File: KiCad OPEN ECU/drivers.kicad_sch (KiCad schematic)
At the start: 52 parts, among them SW5 SW_DPDT_x2, U3 TC4424A, U4 TC4424A, U5 MC33810, U6 MC33810, U7 TC4424A, U8 TC4424A

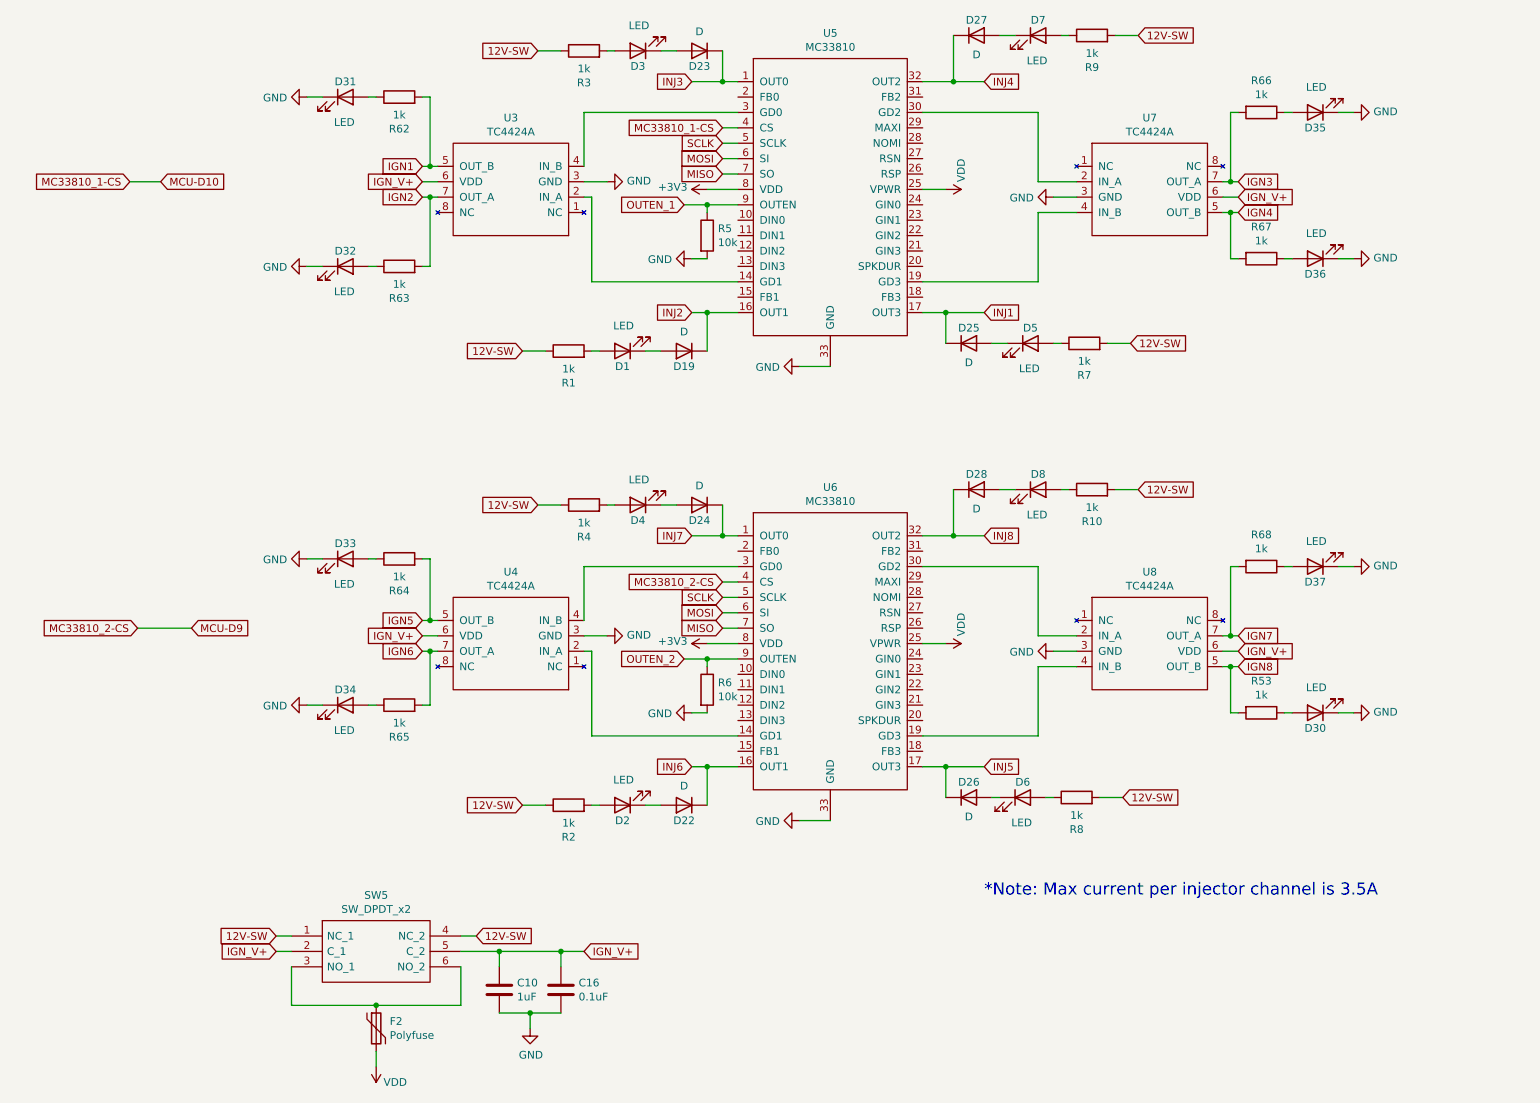
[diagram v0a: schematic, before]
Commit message: Add files via upload
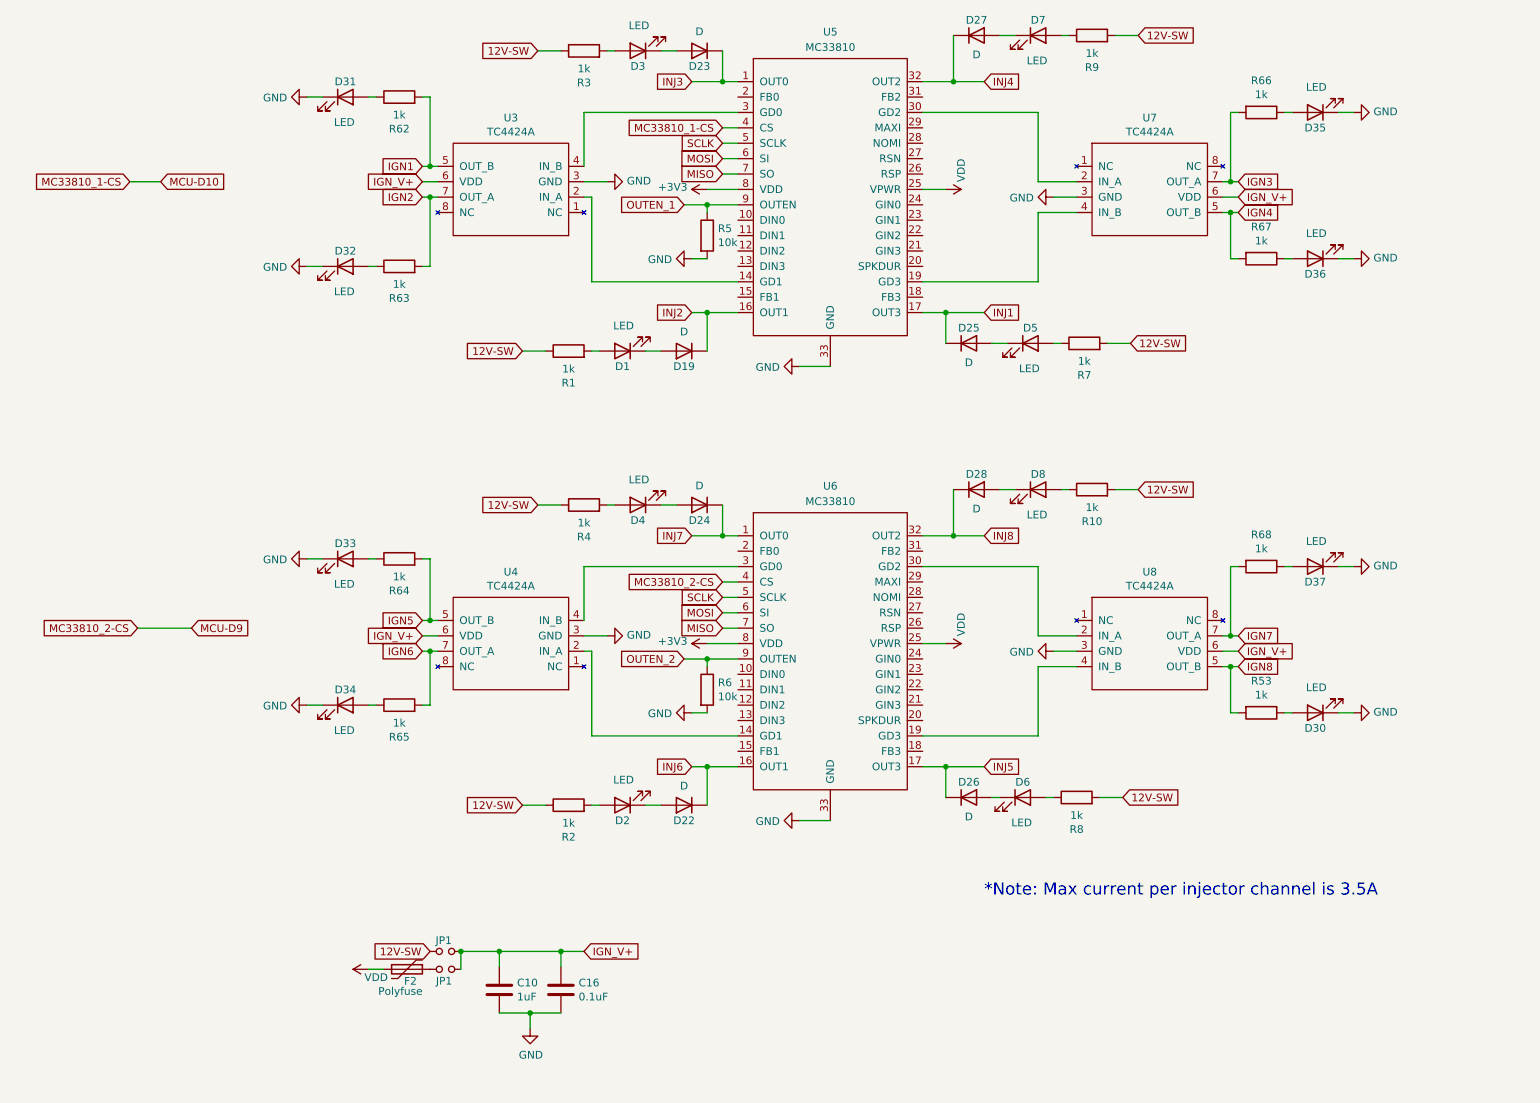
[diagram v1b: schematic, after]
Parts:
- removed SW5: SW_DPDT_x2, Misc:AYZ0202AGRLC, symbol Misc:AYZ0202AGRLC
- removed U5, U6: MC33810, IC_Automotive:SOIC32-P0.65-33N, symbol IC_Automotive:MC33810
- added JP1 (x2): Jumper_NO_Small, Jumper:SolderJumper-2_P1.3mm_Open_Pad1.0x1.5mm, symbol Device:Jumper_NO_Small
- added U5, U6: MC33810, AeonLabs_Automotive:mc33810 SOIC32-P0.65-33N, symbol AeonLabs_Automotive:MC33810
- F2: footprint Fuse:Fuse_1812_4532Metric -> AeonLabs_Power:Fuse_1812_4532Metric
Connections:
- net +3V3: now also U5.8 (VDD), U6.8 (VDD)
- net 12V-SW: now also JP1.1
- net GND: now also U5.33 (GND), U6.33 (GND)
- net IGN_V+: now also JP1.2, JP1.2
- net INJ1: now also U5.17 (OUT3)
- net INJ2: now also U5.16 (OUT1)
- net INJ3: now also U5.1 (OUT0)
- net INJ4: now also U5.32 (OUT2)
- net INJ5: now also U6.17 (OUT3)
- net INJ6: now also U6.16 (OUT1)
- net INJ7: now also U6.1 (OUT0)
- net INJ8: now also U6.32 (OUT2)
- net MC33810_1-CS: now also U5.4 (CS)
- net MC33810_2-CS: now also U6.4 (CS)
- net MISO: now also U5.7 (SO), U6.7 (SO)
- net MOSI: now also U5.6 (SI), U6.6 (SI)
- net OUTEN_1: now also U5.9 (OUTEN)
- net OUTEN_2: now also U6.9 (OUTEN)
- net SCLK: now also U5.5 (SCLK), U6.5 (SCLK)
- net VDD: now also U5.25 (VPWR), U6.25 (VPWR)
- net at U3.2 (IN_A): now also U5.14 (GD1)
- net at U7.4 (IN_B): now also U5.19 (GD3)
- net at U3.4 (IN_B): now also U5.3 (GD0)
- net at U7.2 (IN_A): now also U5.30 (GD2)
- net at U4.2 (IN_A): now also U6.14 (GD1)
- net at U8.4 (IN_B): now also U6.19 (GD3)
- net at U4.4 (IN_B): now also U6.3 (GD0)
- net at U8.2 (IN_A): now also U6.30 (GD2)
- net at F2.1: now also JP1.1
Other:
- moved on the sheet: F2
